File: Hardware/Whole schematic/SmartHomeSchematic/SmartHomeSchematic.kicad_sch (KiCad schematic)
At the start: 6 parts, among them Q1 BC557, SW1 SW_Push

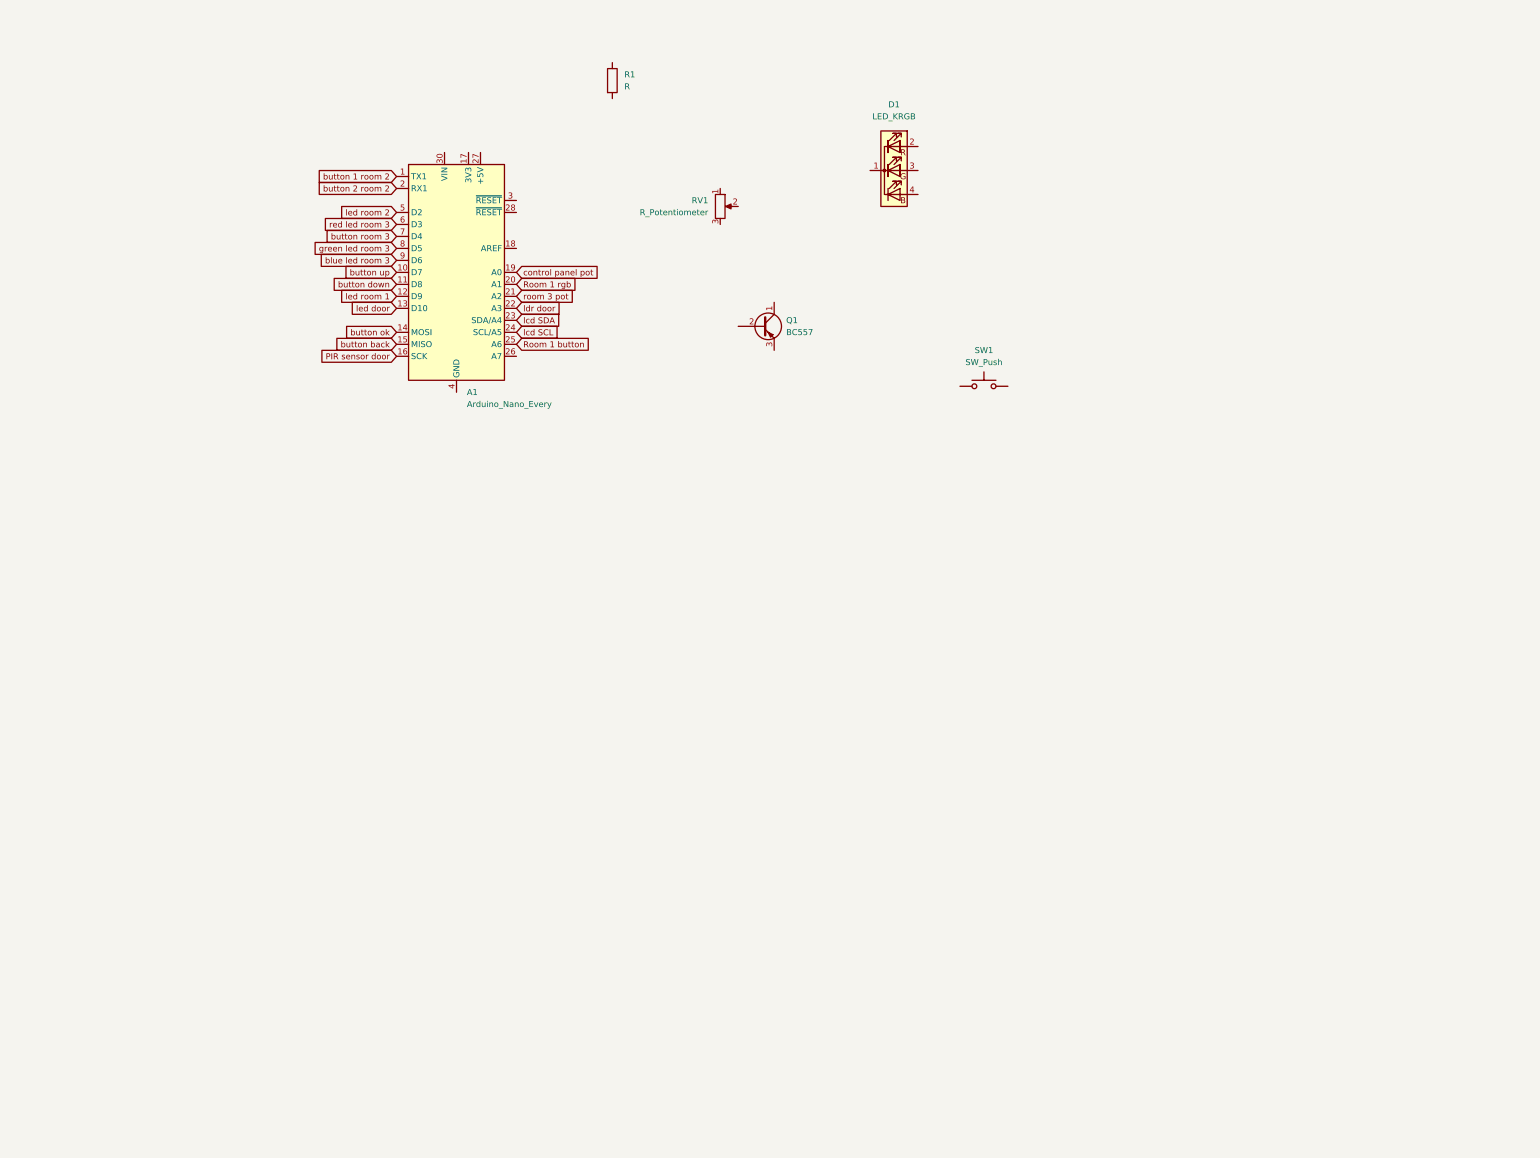
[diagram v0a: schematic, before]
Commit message: Combine partial schematics into one.
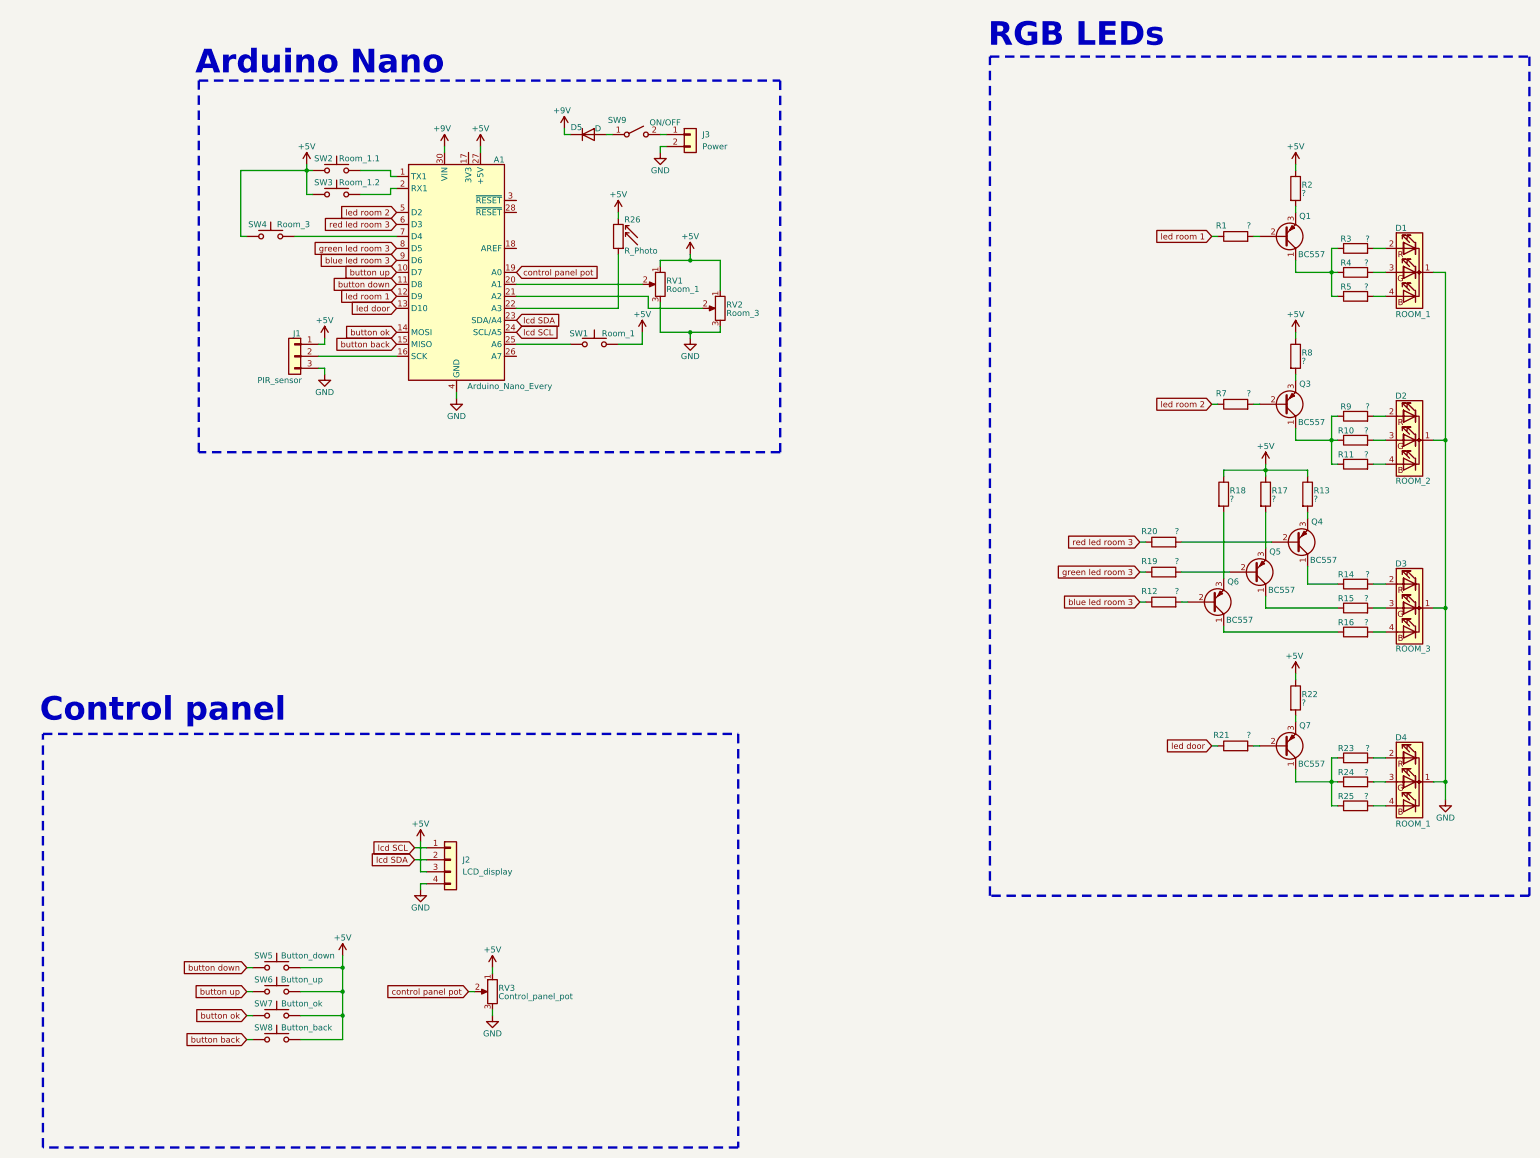
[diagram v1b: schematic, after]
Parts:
- added D2: ROOM_2, symbol Device:LED_KRGB
- added D3: ROOM_3, symbol Device:LED_KRGB
- added D4: ROOM_1, symbol Device:LED_KRGB
- added D5: D, symbol Device:D
- added J1: PIR_sensor, symbol Connector_Generic:Conn_01x03
- added J2: LCD_display, symbol Connector_Generic:Conn_01x04
- added J3: Power, symbol Connector_Generic:Conn_01x02
- added Q3, Q4, Q5, Q6, Q7: BC557, Package_TO_SOT_THT:TO-92_Inline, symbol Transistor_BJT:BC557
- added R10, R11, R12, R13, R14, R15, R16, R17, R18, R19, R2, R20, R21, R22, R23, R24, R25, R3, R4, R5, R7, R8, R9: ?, symbol Device:R
- added R26: R_Photo, symbol Device:R_Photo
- added RV2: Room_3, symbol Device:R_Potentiometer
- added RV3: Control_panel_pot, symbol Device:R_Potentiometer
- added SW2: Room_1.1, symbol Switch:SW_Push
- added SW3: Room_1.2, symbol Switch:SW_Push
- added SW4: Room_3, symbol Switch:SW_Push
- added SW5: Button_down, symbol Switch:SW_Push
- added SW6: Button_up, symbol Switch:SW_Push
- added SW7: Button_ok, symbol Switch:SW_Push
- added SW8: Button_back, symbol Switch:SW_Push
- added SW9: ON/OFF, symbol Switch:SW_SPST
- D1: value LED_KRGB -> ROOM_1
- R1: value R -> ?
- RV1: value R_Potentiometer -> Room_1
- SW1: value SW_Push -> Room_1
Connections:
- net Room 1 button is gone; now on an unnamed net: A1.25 (A6)
- net Room 1 rgb is gone; now on an unnamed net: A1.20 (A1)
- net blue led room 3: now also R12.1
- net button back: now also SW8.1
- net button down: now also SW5.1
- net button ok: now also SW7.1
- net button up: now also SW6.1
- net control panel pot: now also RV3.2
- net green led room 3: now also R19.1
- net lcd SCL: now also J2.1 (Pin_1)
- net lcd SDA: now also J2.2 (Pin_2)
- net led door: now also R21.1
- net led room 1: now also R1.1
- net led room 2: now also R7.1
- net red led room 3: now also R20.1
- net +5V: now reaches SW1.2
- net +5V: now also A1.27 (+5V), RV1.1, J1.1 (Pin_1), J2.3 (Pin_3), R13.1, R17.1, R18.1, R2.1, R22.1, R26.2, R8.1, RV2.1, RV3.1, SW2.1, SW3.1, SW4.1, SW5.2, SW6.2, SW7.2, SW8.2
- net at Q1.1 (C): now also R3.1, R4.1, R5.1
- net at Q1.2 (B): now also R1.2
- net at Q1.3 (E): now also R2.2
- net GND: now reaches D1.1 (K)
- net GND: now also A1.29 (GND), A1.4 (GND), RV1.3, D2.1 (K), D3.1 (K), D4.1 (K), J1.3 (Pin_3), J2.4 (Pin_4), J3.2 (Pin_2), RV2.3, RV3.3
- net at D1.2 (RA): now also R3.2
- net at D1.3 (GA): now also R4.2
- net at D1.4 (BA): now also R5.2
- net +9V: now reaches A1.30 (VIN)
- net +9V: now also D5.1 (K)
- net PIR sensor door: no longer names the net of A1.16 (SCK)
- net PIR sensor door: now also J1.2 (Pin_2)
- net button 1 room 2: no longer names the net of A1.1 (TX1)
- net button 1 room 2: now also SW2.2
- net button 2 room 2: no longer names the net of A1.2 (RX1)
- net button 2 room 2: now also SW3.2
- net button room 3: no longer names the net of A1.7 (D4)
- net button room 3: now also SW4.2
- net ldr door: no longer names the net of A1.22 (A3)
- net ldr door: now also R26.1
- net room 3 pot: no longer names the net of A1.21 (A2)
- net room 3 pot: now also RV2.2
- new net: Q6.1 (C), R16.1
- new net: D3.4 (BA), R16.2
- new net: Q6.2 (B), R12.2
- new net: J3.1 (Pin_1), SW9.2 (B)
- new net: Q5.1 (C), R15.1
- new net: D3.3 (GA), R15.2
- new net: Q3.3 (E), R8.2
- new net: Q3.1 (C), R10.1, R11.1, R9.1
- new net: D2.2 (RA), R9.2
- new net: D2.3 (GA), R10.2
- new net: D2.4 (BA), R11.2
- new net: Q7.1 (C), R23.1, R24.1, R25.1
- new net: D4.4 (BA), R25.2
- new net: D3.2 (RA), R14.2
- new net: Q7.2 (B), R21.2
- new net: Q7.3 (E), R22.2
- new net: D4.2 (RA), R23.2
- new net: Q5.2 (B), R19.2
- new net: Q4.1 (C), R14.1
- new net: Q6.3 (E), R18.2
- new net: Q5.3 (E), R17.2
- new net: Q3.2 (B), R7.2
- new net: Q4.2 (B), R20.2
- new net: Q4.3 (E), R13.2
- new net: D4.3 (GA), R24.2
- new net: D5.2 (A), SW9.1 (A)
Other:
- note added: "Arduino Nano"
- note added: "Control panel"
- note added: "RGB LEDs"
- company: (none) -> Group 7
- title: (none) -> Smart home model
- moved on the sheet: D1, Q1, R1, RV1, SW1
